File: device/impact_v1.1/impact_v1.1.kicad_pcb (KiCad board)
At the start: 4 copper layers, 32.3 x 27 mm, 24 parts, among them U1 ESP32-WROOM-32, U2 MIC5200-3.3BM-TR, U3 ADXL375BCCZ, U4 MPU-6050

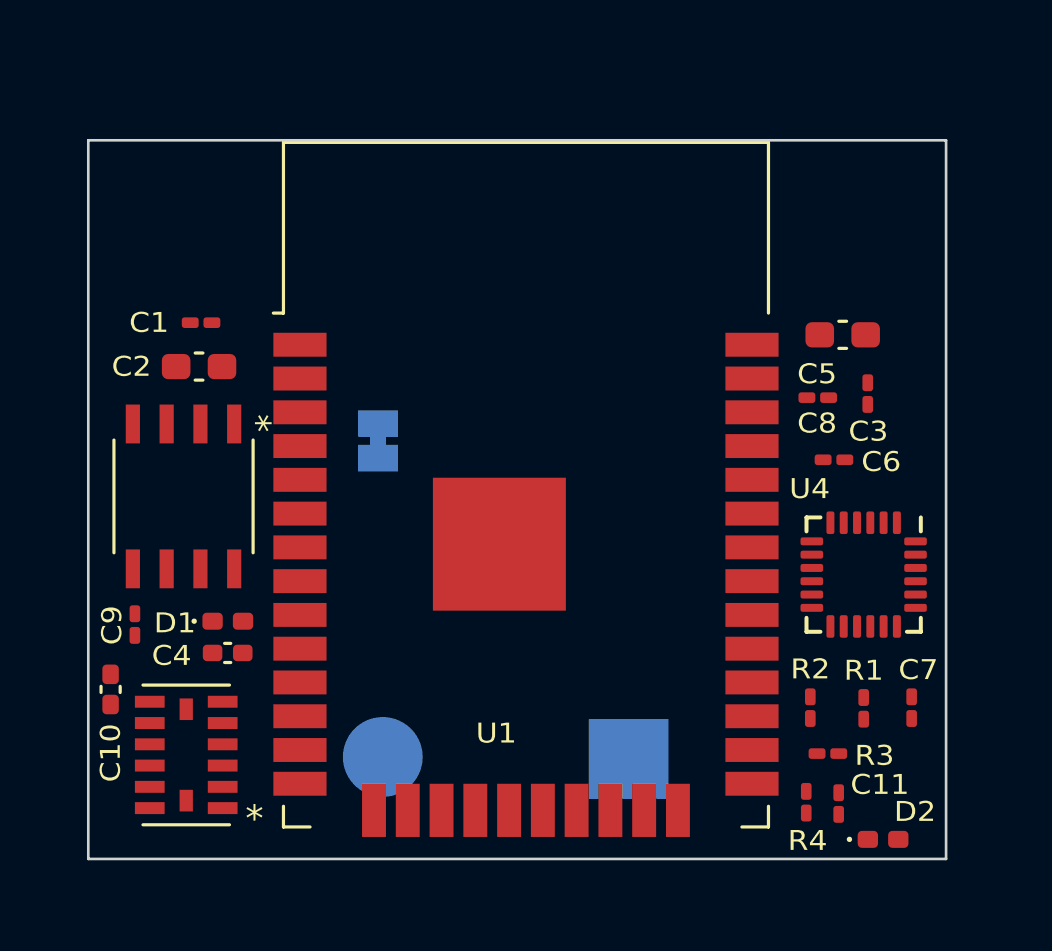
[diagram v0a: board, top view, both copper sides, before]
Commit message: LSV v1.1
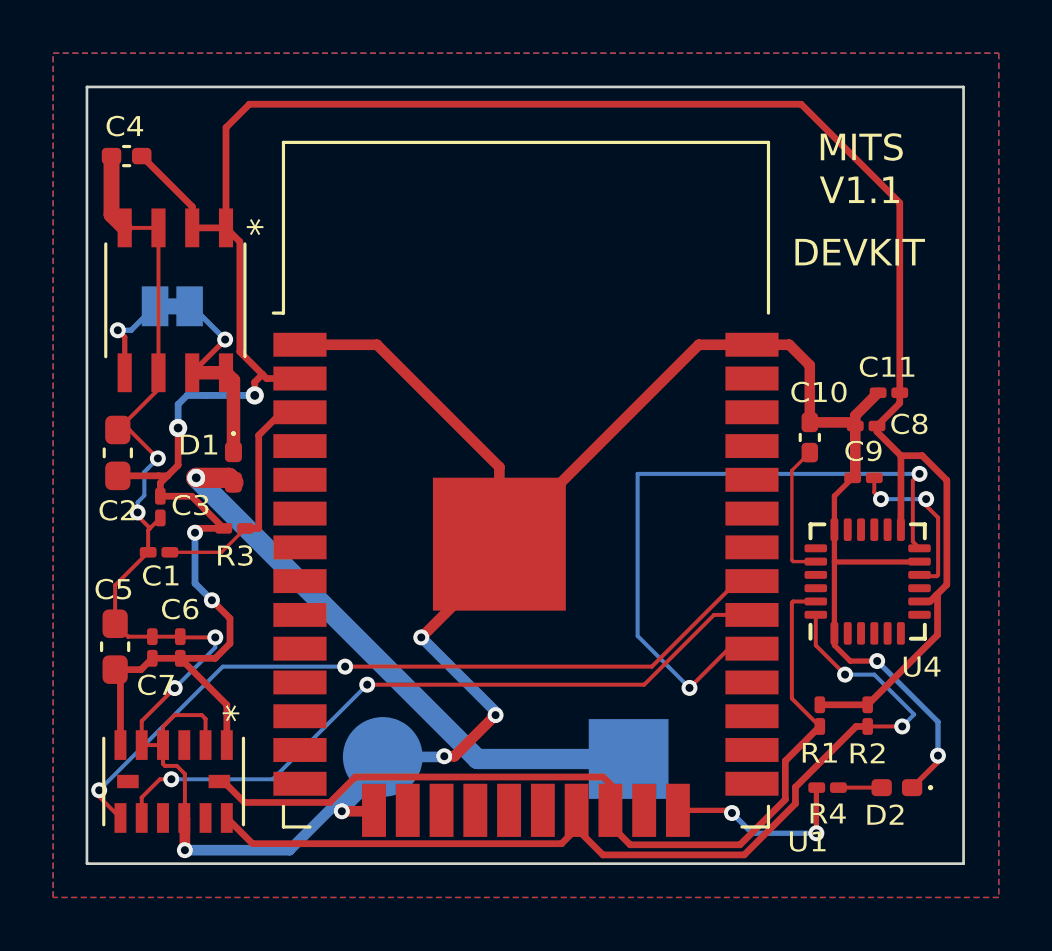
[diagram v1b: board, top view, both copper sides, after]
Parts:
- moved C5 29.8 mm to (136.9, 97.2), turned to -90 degrees
- moved C7 28.6 mm to (138.3, 97.3), turned to -90 degrees
- moved C10 27.9 mm to (163.1, 89.4)
- moved C9 27.9 mm to (165.1, 90.9), turned to 180 degrees
- moved C3 26.9 mm to (138.7, 92.0), turned to -90 degrees
- moved C6 25.6 mm to (139.4, 97.3), turned to 90 degrees
- moved R3 23.9 mm to (141.4, 92.8), turned to 0 degrees
- moved C4 19.1 mm to (137.4, 78.8)
- moved C11 15.6 mm to (166.1, 87.7), turned to 180 degrees
- moved JP1 9.24 mm to (139.1, 84.5), turned to 180 degrees
- moved C1 8.78 mm to (138.6, 93.7)
- moved U2 7.38 mm to (139.2, 84.2)
- moved D1 5.80 mm to (141.4, 90.5), turned to -90 degrees
- moved C2 4.46 mm to (137.1, 90.0), turned to 90 degrees
- moved R2 2.18 mm to (165.2, 99.8), turned to -90 degrees
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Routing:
- net GND: track 0.00 -> 119.4 mm, vias 0 -> 11
- net VDD: track 0.00 -> 100.6 mm, vias 0 -> 4
- net SDA1: track 0.00 -> 36.1 mm, vias 0 -> 2
- net SCL1: track 0.00 -> 34.0 mm
- net INT1: track 0.00 -> 29.2 mm, vias 0 -> 2
- net INT2: track 0.00 -> 26.6 mm, vias 0 -> 2
- net INT3: track 0.00 -> 25.4 mm, vias 0 -> 2
- net +BATT: track 0.00 -> 22.1 mm, vias 0 -> 1
- net Net-(C1-Pad1): track 0.00 -> 9.12 mm
- net Net-(D1-Pad1): track 0.00 -> 7.98 mm, vias 0 -> 1
- net Net-(U1-Pad24): track 0.00 -> 7.29 mm, vias 0 -> 2
- net Net-(C9-Pad1): track 0.00 -> 6.38 mm, vias 0 -> 2
- net Net-(C10-Pad1): track 0.00 -> 5.25 mm
- net Net-(JP1-Pad2): track 0.00 -> 3.48 mm, vias 0 -> 1
- net Net-(D2-Pad2): track 0.00 -> 1.63 mm
- added copper zone on B.Cu, net (none)
- added copper zone on F.Cu, net GND
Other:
- board size 32.3 x 27 mm -> 33 x 29.2 mm
- copper layers 4 -> 2
- rule solder_mask_min_width: 0.1016 -> 0.12
- board text added: "DEVKIT"
- board text added: "MITS V1.1"
- board text added: "Property of Amogh Kashyap"
